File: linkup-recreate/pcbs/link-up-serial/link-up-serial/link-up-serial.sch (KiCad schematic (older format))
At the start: 6 parts

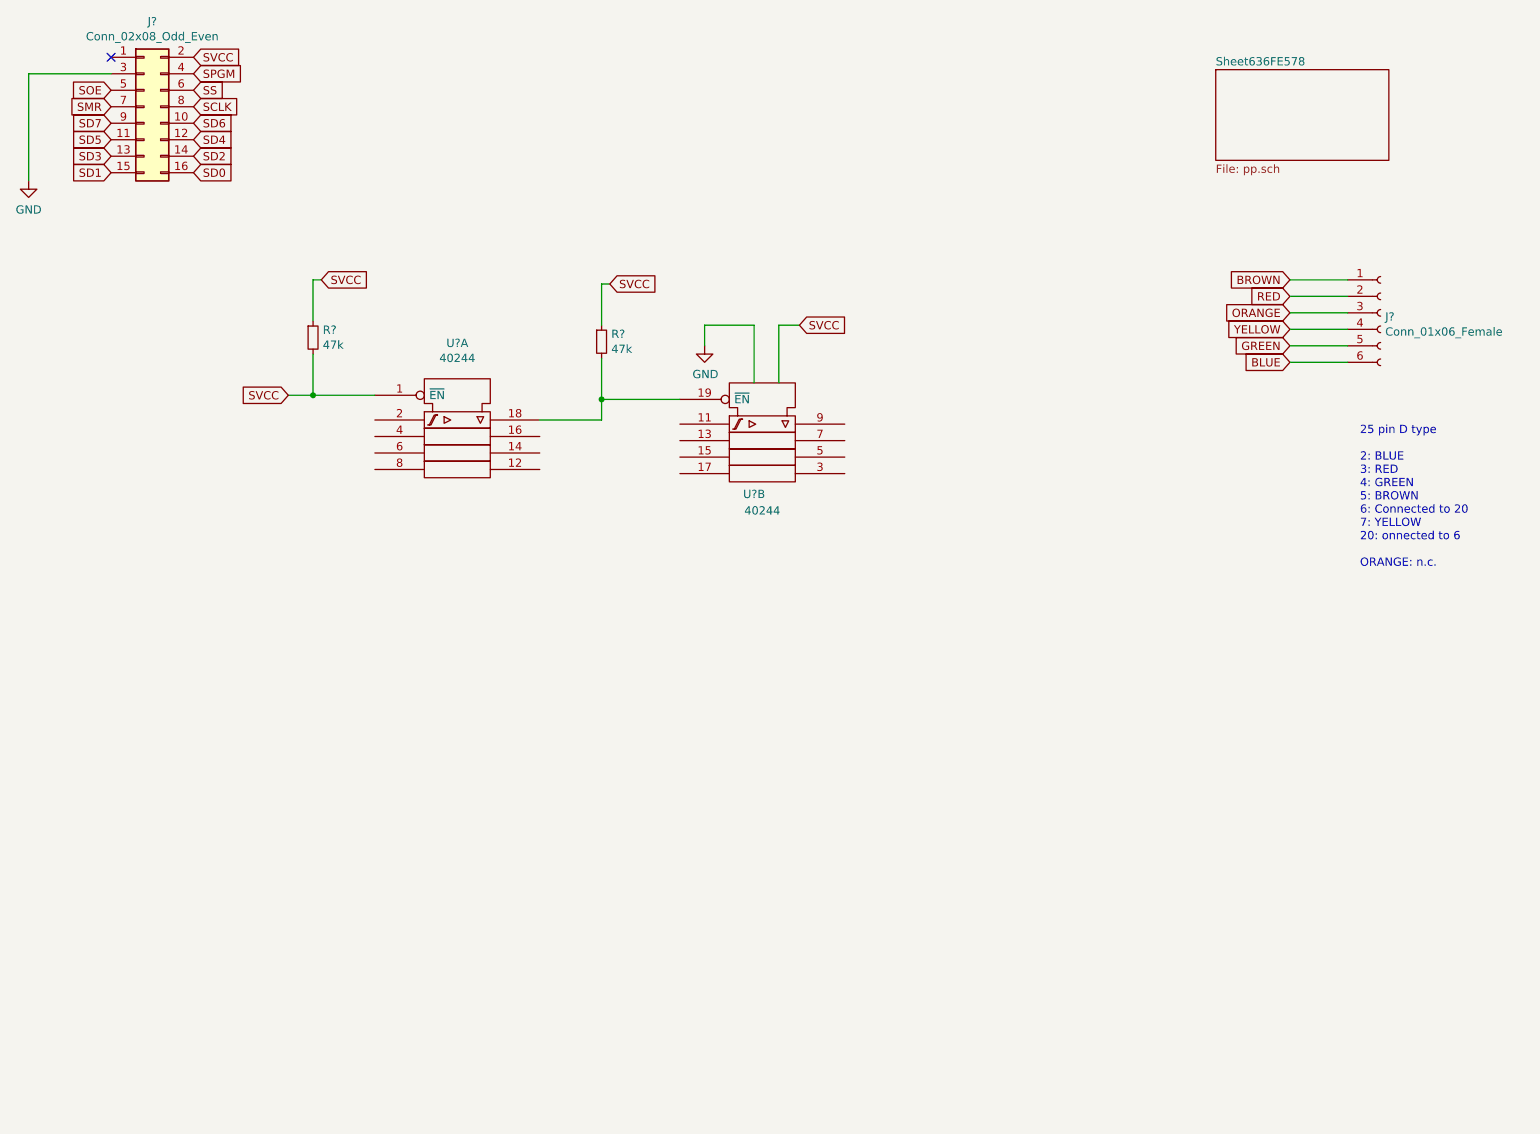
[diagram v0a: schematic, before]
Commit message: Updates
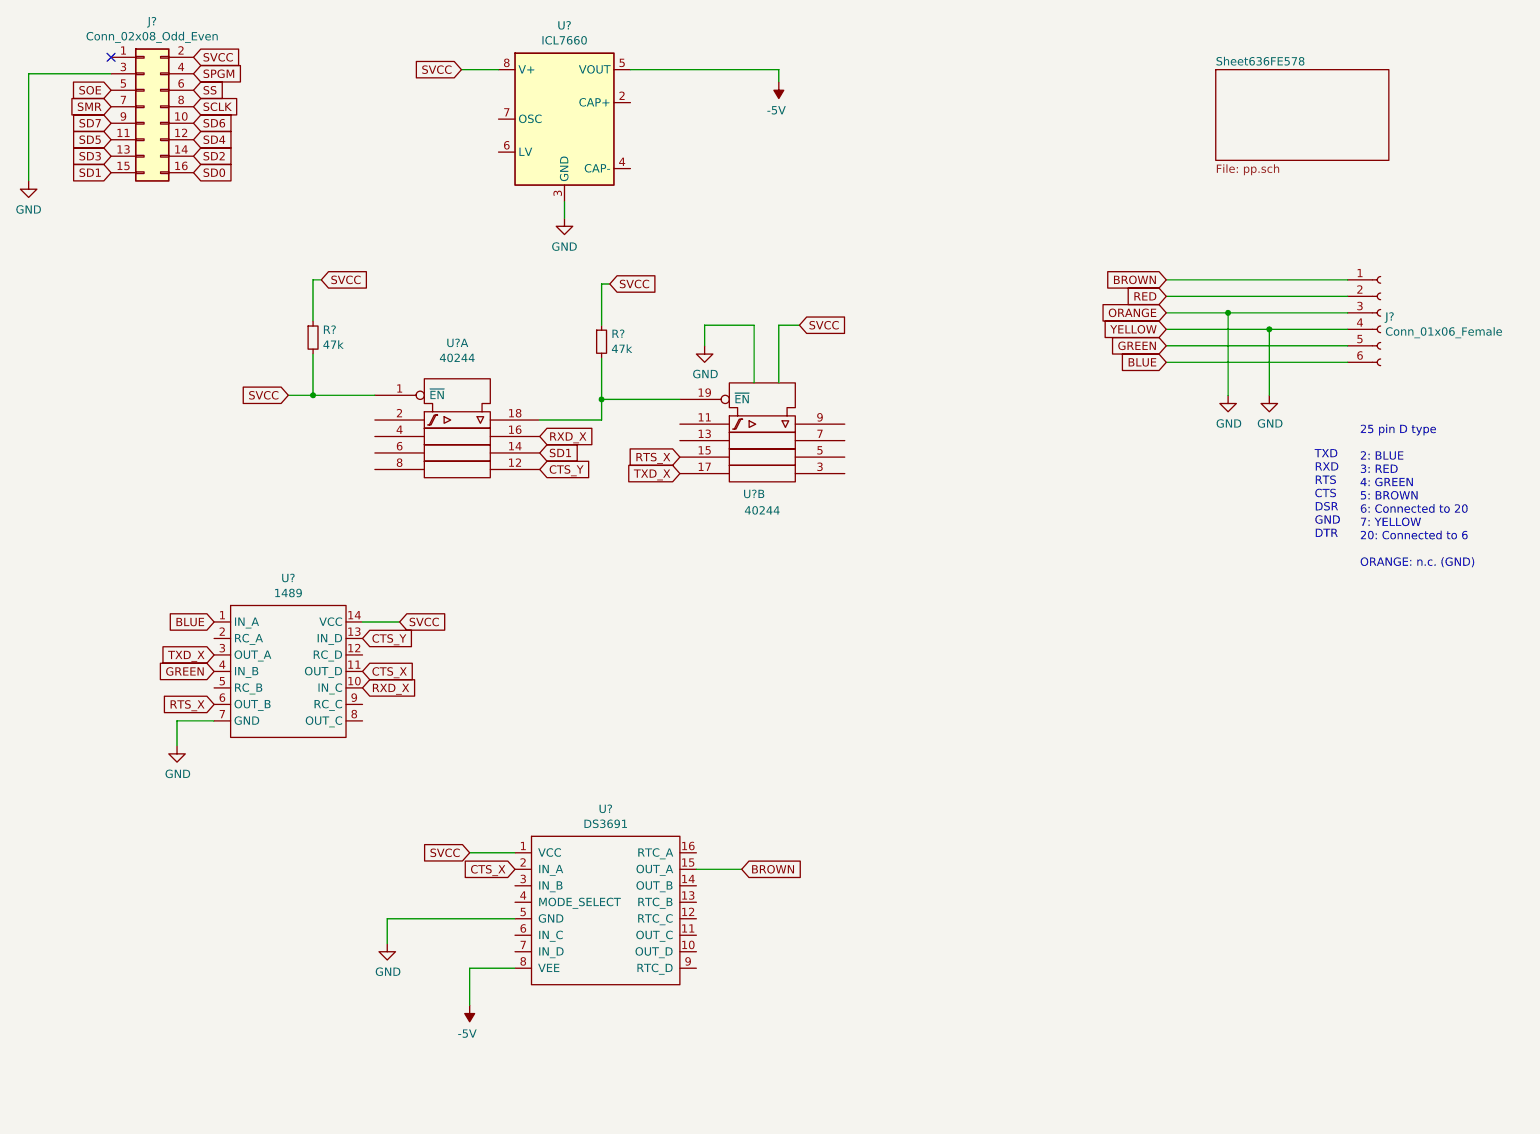
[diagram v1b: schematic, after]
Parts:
- added U?: 1489, symbol ajm:1489
- added U?: DS3691, symbol ajm:DS3691
- added U?: ICL7660, symbol Regulator_SwitchedCapacitor:ICL7660
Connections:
- net ORANGE is gone; now on net GND: J?.3 (Pin_3)
- net YELLOW is gone; now on net GND: J?.4 (Pin_4)
- net BLUE: now also U?.1 (IN_A)
- net BROWN: now also U?.15 (OUT_A)
- net GND: now also U?.3 (GND), U?.5 (GND), U?.7 (GND)
- net GREEN: now also U?.4 (IN_B)
- net SD1: now also U?.14
- net Vdd: now also U?.1 (VCC), U?.14 (VCC), U?.8 (V+)
- net CTS_Y: now reaches U?.12
- net CTS_Y: now also U?.13 (IN_D)
- net RXD_X: now reaches U?.16
- net RXD_X: now also U?.10 (IN_C)
- net RTS_X: now reaches U?.15
- net RTS_X: now also U?.6 (OUT_B)
- net TXD_X: now reaches U?.17
- net TXD_X: now also U?.3 (OUT_A)
- new net -5V: U?.5 (VOUT), U?.8 (VEE)
- new net CTS_X: U?.11 (OUT_D), U?.2 (IN_A)
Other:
- note added: "25 pin D type\n\n2: BLUE\n3: RED\n4: GREEN\n5: BROWN\n6: Connected to 20\n7: YELLOW\n20: Connected to 6\n\nORANGE: n.c. (GND)\n"
- note added: "TXD\nRXD\nRTS\nCTS\nDSR\nGND\nDTR"
- note removed: "25 pin D type\n\n2: BLUE\n3: RED\n4: GREEN\n5: BROWN\n6: Connected to 20\n7: YELLOW\n20: onnected to 6\n\nORANGE: n.c.\n"
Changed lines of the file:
@@
 Wire Wire Line
 	2700 2425 2750 2425
-Text GLabel 8625 2425 0    50   Input ~ 0
+Text GLabel 7875 2425 0    50   Input ~ 0
 BROWN
-Text GLabel 8625 2525 0    50   Input ~ 0
+Text GLabel 7875 2525 0    50   Input ~ 0
 RED
-Text GLabel 8625 2625 0    50   Input ~ 0
+Text GLabel 7875 2625 0    50   Input ~ 0
 ORANGE
-Text GLabel 8625 2725 0    50   Input ~ 0
+Text GLabel 7875 2725 0    50   Input ~ 0
 YELLOW
-Text GLabel 8625 2825 0    50   Input ~ 0
+Text GLabel 7875 2825 0    50   Input ~ 0
 GREEN
-Text GLabel 8625 2925 0    50   Input ~ 0
+Text GLabel 7875 2925 0    50   Input ~ 0
 BLUE
 $Comp
@@
 $EndComp
 Wire Wire Line
-	8975 2425 8625 2425
-Wire Wire Line
-	8625 2525 8975 2525
-Wire Wire Line
-	8975 2625 8625 2625
-Wire Wire Line
-	8625 2725 8975 2725
-Wire Wire Line
-	8625 2825 8975 2825
-Wire Wire Line
-	8625 2925 8975 2925
+	8975 2425 7875 2425
+Wire Wire Line
+	7875 2525 8975 2525
+Wire Wire Line
+	8975 2625 8250 2625
+Wire Wire Line
+	7875 2725 8500 2725
+Wire Wire Line
+	7875 2825 8975 2825
+Wire Wire Line
+	7875 2925 8975 2925
 Text Notes 9050 4175 0    50   ~ 0
-25 pin D type\n\n2: BLUE\n3: RED\n4: GREEN\n5: BROWN\n6: Connected to 20\n7: YELLOW\n20: onnected to 6\n\nORANGE: n.c.\n
+25 pin D type\n\n2: BLUE\n3: RED\n4: GREEN\n5: BROWN\n6: Connected to 20\n7: YELLOW\n20: Connected to 6\n\nORANGE: n.c. (GND)\n
 Wire Wire Line
 	4075 3275 4450 3275
@@
 	4925 3150 4450 3150
 Connection ~ 4450 3150
+$Comp
+L ajm:1489 U?
+U 1 1 6371CD69
+P 2050 4400
+F 0 "U?" H 2550 4565 50  0000 C CNN
+F 1 "1489" H 2550 4474 50  0000 C CNN
+F 2 "" H 2050 4400 50  0001 C CNN
+F 3 "" H 2050 4400 50  0001 C CNN
+	1    2050 4400
+	1    0    0    -1
+$EndComp
+$Comp
+L ajm:DS3691 U?
+U 1 1 6371DF57
+P 4025 5800
+F 0 "U?" H 4475 5965 50  0000 C CNN
+F 1 "DS3691" H 4475 5874 50  0000 C CNN
+F 2 "" H 4025 5800 50  0001 C CNN
+F 3 "" H 4025 5800 50  0001 C CNN
+	1    4025 5800
+	1    0    0    -1
+$EndComp
+$Comp
+L Regulator_SwitchedCapacitor:ICL7660 U?
+U 1 1 6371F6A3
+P 4225 1450
+F 0 "U?" H 4225 2017 50  0000 C CNN
+F 1 "ICL7660" H 4225 1926 50  0000 C CNN
+F 2 "" H 4325 1350 50  0001 C CNN
+F 3 "http://datasheets.maximintegrated.com/en/ds/ICL7660-MAX1044.pdf" H 4325 1350 50  0001 C CNN
+	1    4225 1450
+	1    0    0    -1
+$EndComp
+Text GLabel 3600 1150 0    50   Input ~ 0
+SVCC
+Wire Wire Line
+	3600 1150 3825 1150
+$Comp
+L power:GND #PWR?
+U 1 1 63721337
+P 4225 2050
+AR Path="/6104FF77/63721337" Ref="#PWR?"  Part="1"
+AR Path="/63721337" Ref="#PWR?"  Part="1"
+AR Path="/636FE579/63721337" Ref="#PWR?"  Part="1"
+F 0 "#PWR?" H 4225 1800 50  0001 C CNN
+F 1 "GND" H 4225 1875 50  0000 C CNN
+F 2 "" H 4225 2050 50  0001 C CNN
+F 3 "" H 4225 2050 50  0001 C CNN
+	1    4225 2050
+	1    0    0    -1
+$EndComp
+Wire Wire Line
+	4225 2050 4225 1950
+$Comp
+L power:-5V #PWR?
+U 1 1 63721F90
+P 5525 1225
+F 0 "#PWR?" H 5525 1325 50  0001 C CNN
+F 1 "-5V" H 5540 1398 50  0000 C CNN
+F 2 "" H 5525 1225 50  0001 C CNN
+F 3 "" H 5525 1225 50  0001 C CNN
+	1    5525 1225
+	-1   0    0    1
+$EndComp
+$Comp
+L power:-5V #PWR?
+U 1 1 63722CFC
+P 3650 6825
+F 0 "#PWR?" H 3650 6925 50  0001 C CNN
+F 1 "-5V" H 3665 6998 50  0000 C CNN
+F 2 "" H 3650 6825 50  0001 C CNN
+F 3 "" H 3650 6825 50  0001 C CNN
+	1    3650 6825
+	-1   0    0    1
+$EndComp
+Wire Wire Line
+	3925 6600 3650 6600
+Wire Wire Line
+	3650 6600 3650 6825
+Wire Wire Line
+	5525 1150 5525 1225
+Wire Wire Line
+	4625 1150 5525 1150
+Wire Wire Line
+	3925 5900 3650 5900
+$Comp
+L power:GND #PWR?
+U 1 1 63725A73
+P 3150 6450
+F 0 "#PWR?" H 3150 6200 50  0001 C CNN
+F 1 "GND" H 3155 6277 50  0000 C CNN
+F 2 "" H 3150 6450 50  0001 C CNN
+F 3 "" H 3150 6450 50  0001 C CNN
+	1    3150 6450
+	1    0    0    -1
+$EndComp
+Wire Wire Line
+	3925 6300 3150 6300
+Wire Wire Line
+	3150 6300 3150 6450
+Text GLabel 5300 6000 2    50   Input ~ 0
+BROWN
+Wire Wire Line
+	5300 6000 5025 6000
+Text GLabel 4925 3600 0    50   Input ~ 0
+TXD_X
+Text GLabel 2100 4700 0    50   Input ~ 0
+TXD_X
+$Comp
+L power:GND #PWR?
+U 1 1 63727763
+P 1875 5250
+F 0 "#PWR?" H 1875 5000 50  0001 C CNN
+F 1 "GND" H 1880 5077 50  0000 C CNN
+F 2 "" H 1875 5250 50  0001 C CNN
+F 3 "" H 1875 5250 50  0001 C CNN
+	1    1875 5250
+	1    0    0    -1
+$EndComp
+Wire Wire Line
+	2100 5100 1875 5100
+Wire Wire Line
+	1875 5100 1875 5250
+Text GLabel 3650 5900 0    50   Input ~ 0
+SVCC
+Text GLabel 3225 4500 2    50   Input ~ 0
+SVCC
+Wire Wire Line
+	3000 4500 3225 4500
+Text GLabel 2100 4500 0    50   Input ~ 0
+BLUE
+Text Notes 8775 4000 0    50   ~ 0
+TXD\nRXD\nRTS\nCTS\nDSR\nGND\nDTR
+$Comp
+L power:GND #PWR?
+U 1 1 6372AA19
+P 8250 3125
+F 0 "#PWR?" H 8250 2875 50  0001 C CNN
+F 1 "GND" H 8255 2952 50  0000 C CNN
+F 2 "" H 8250 3125 50  0001 C CNN
+F 3 "" H 8250 3125 50  0001 C CNN
+	1    8250 3125
+	1    0    0    -1
+$EndComp
+Wire Wire Line
+	8250 3125 8250 2625
+Connection ~ 8250 2625
+Wire Wire Line
+	8250 2625 7875 2625
+$Comp
+L power:GND #PWR?
+U 1 1 6372B87A
+P 8500 3125
+F 0 "#PWR?" H 8500 2875 50  0001 C CNN
+F 1 "GND" H 8505 2952 50  0000 C CNN
+F 2 "" H 8500 3125 50  0001 C CNN
+F 3 "" H 8500 3125 50  0001 C CNN
+	1    8500 3125
+	1    0    0    -1
+$EndComp
+Wire Wire Line
+	8500 3125 8500 2725
+Connection ~ 8500 2725
+Wire Wire Line
+	8500 2725 8975 2725
+Text GLabel 4075 3375 2    50   Input ~ 0
+RXD_X
+Text GLabel 3000 4900 2    50   Input ~ 0
+RXD_X
+Text GLabel 2100 4800 0    50   Input ~ 0
+GREEN
+Text GLabel 2100 5000 0    50   Input ~ 0
+RTS_X
+Text GLabel 4925 3500 0    50   Input ~ 0
+RTS_X
+Text GLabel 4075 3475 2    50   Input ~ 0
+SD1
+Text GLabel 4075 3575 2    50   Input ~ 0
+CTS_Y
+Text GLabel 3000 4800 2    50   Input ~ 0
+CTS_X
+Text GLabel 3925 6000 0    50   Input ~ 0
+CTS_X
+Text GLabel 3000 4600 2    50   Input ~ 0
+CTS_Y
 $EndSCHEMATC

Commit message: Updates
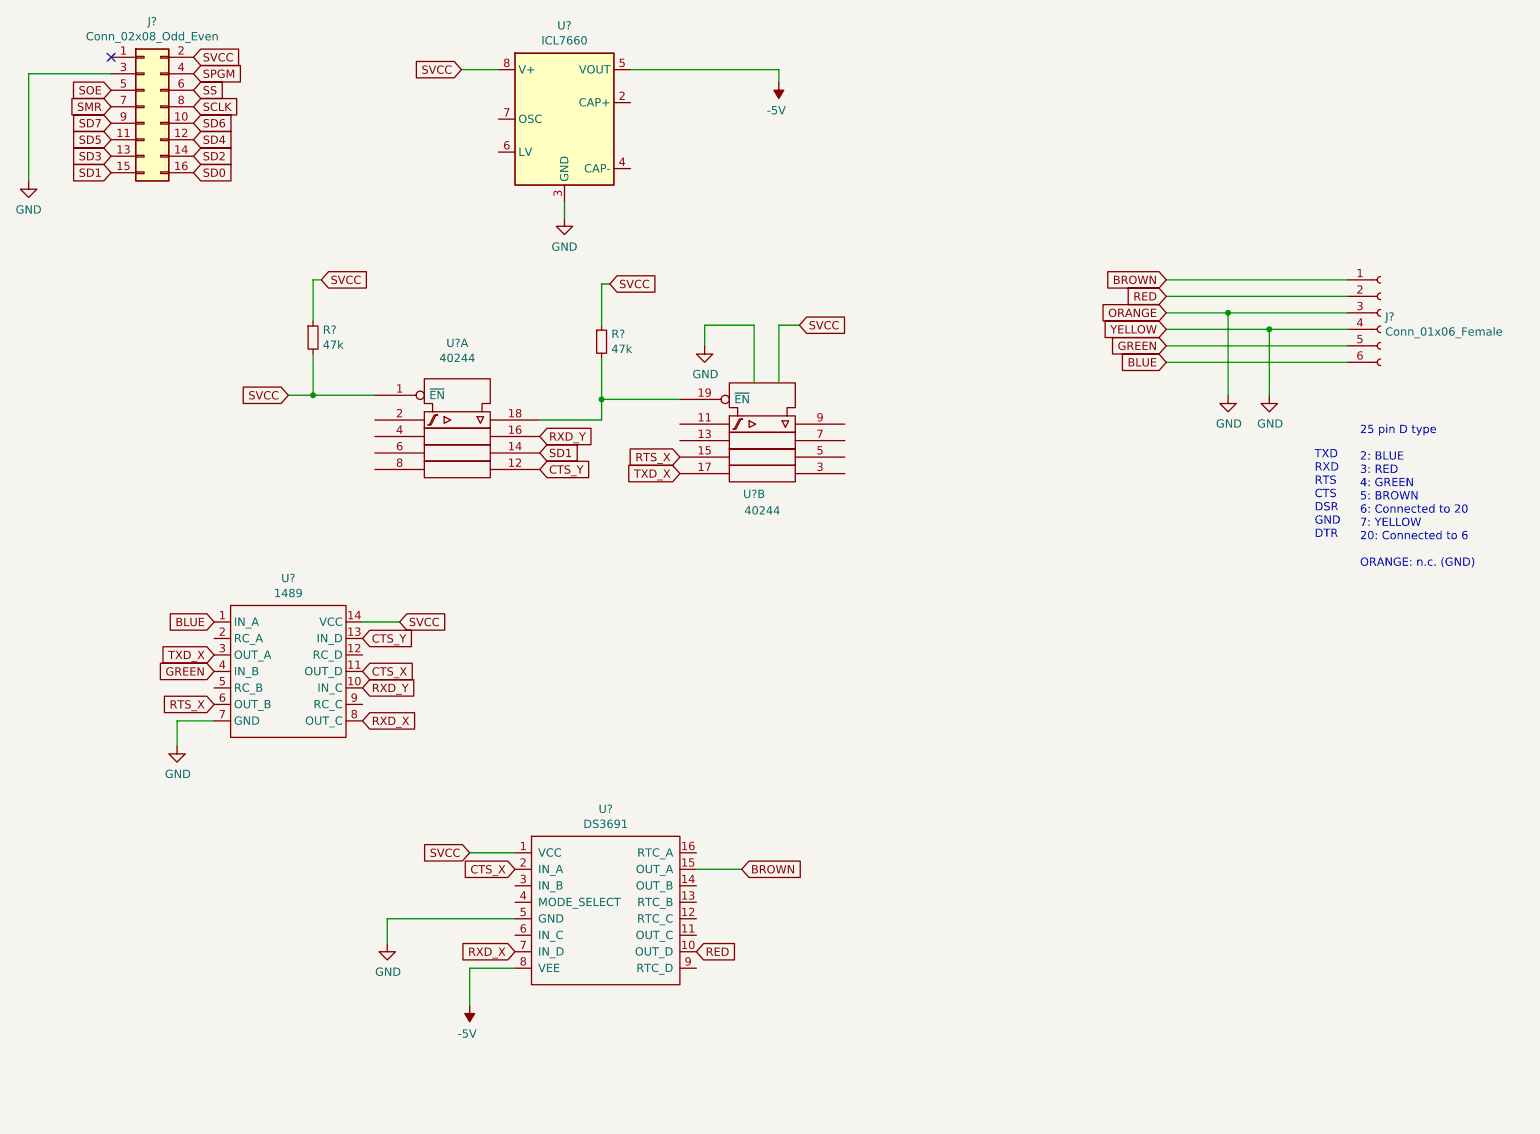
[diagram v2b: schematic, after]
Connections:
- net RED: now also U?.10 (OUT_D)
- net RXD_X: now also U?.7 (IN_D), U?.8 (OUT_C); no longer U?.10 (IN_C), U?.16
- new net RXD_Y: U?.10 (IN_C), U?.16
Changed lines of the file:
@@
 $Descr A4 11693 8268
 encoding utf-8
-Sheet 1 2
+Sheet 1 1
 Title ""
 Date ""
@@
 Comment4 ""
 $EndDescr
-$Sheet
-S 8175 1150 1050 550
-U 636FE579
-F0 "Sheet636FE578" 50
-F1 "pp.sch" 50
-$EndSheet
 Text GLabel 1475 1775 0    50   Input ~ 0
 SD1
@@
 	8500 2725 8975 2725
 Text GLabel 4075 3375 2    50   Input ~ 0
-RXD_X
+RXD_Y
 Text GLabel 3000 4900 2    50   Input ~ 0
-RXD_X
+RXD_Y
 Text GLabel 2100 4800 0    50   Input ~ 0
 GREEN
@@
 Text GLabel 3000 4600 2    50   Input ~ 0
 CTS_Y
+Text GLabel 3000 5100 2    50   Input ~ 0
+RXD_X
+Text GLabel 3925 6500 0    50   Input ~ 0
+RXD_X
+Text GLabel 5025 6500 2    50   Input ~ 0
+RED
 $EndSCHEMATC

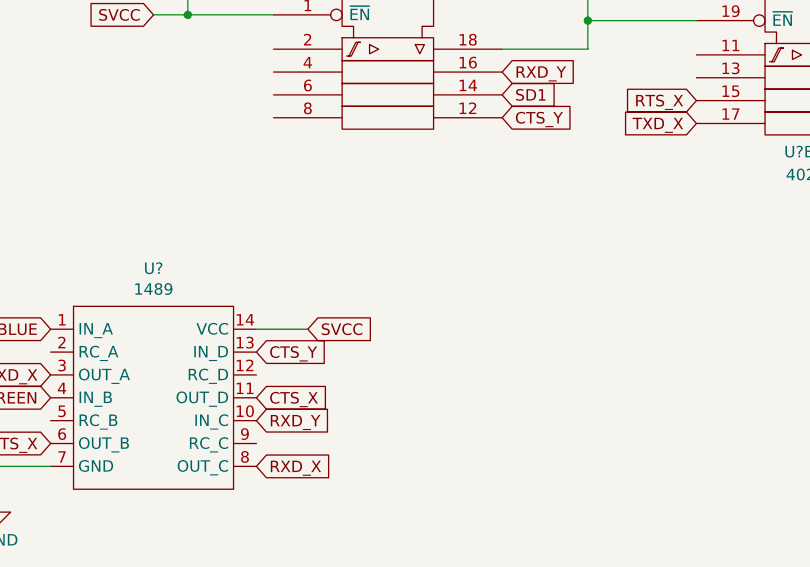
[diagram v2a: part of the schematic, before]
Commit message: Updates
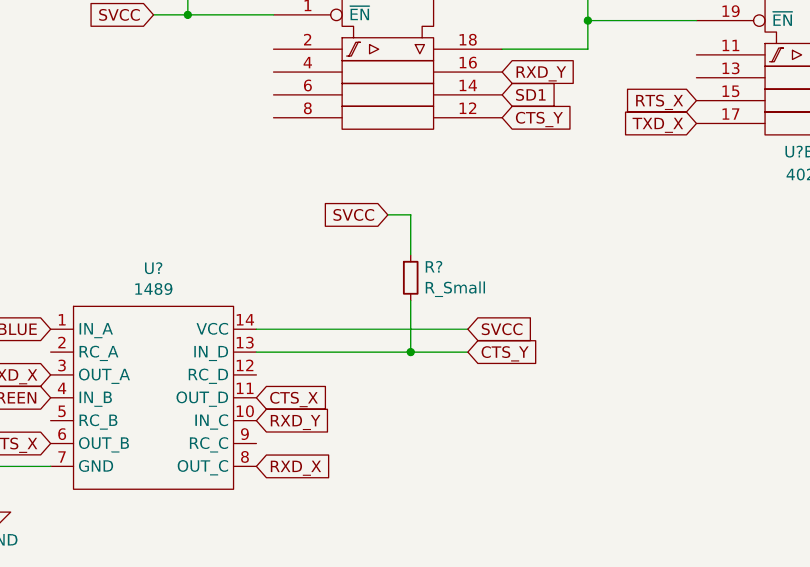
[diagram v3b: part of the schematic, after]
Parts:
- added R?: R_Small, symbol Device:R_Small
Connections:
- net CTS_Y: now also R?.2
- net Vdd: now also R?.1
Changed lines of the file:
@@
 Text GLabel 3650 5900 0    50   Input ~ 0
 SVCC
-Text GLabel 3225 4500 2    50   Input ~ 0
+Text GLabel 3925 4500 2    50   Input ~ 0
 SVCC
-Wire Wire Line
-	3000 4500 3225 4500
 Text GLabel 2100 4500 0    50   Input ~ 0
 BLUE
@@
 Text GLabel 3925 6000 0    50   Input ~ 0
 CTS_X
-Text GLabel 3000 4600 2    50   Input ~ 0
+Text GLabel 3925 4600 2    50   Input ~ 0
 CTS_Y
 Text GLabel 3000 5100 2    50   Input ~ 0
@@
 Text GLabel 5025 6500 2    50   Input ~ 0
 RED
+Wire Wire Line
+	3000 4600 3675 4600
+Wire Wire Line
+	3000 4500 3925 4500
+$Comp
+L Device:R_Small R?
+U 1 1 637324DD
+P 3675 4275
+F 0 "R?" H 3734 4321 50  0000 L CNN
+F 1 "R_Small" H 3734 4230 50  0000 L CNN
+F 2 "" H 3675 4275 50  0001 C CNN
+F 3 "~" H 3675 4275 50  0001 C CNN
+	1    3675 4275
+	1    0    0    -1
+$EndComp
+Text GLabel 3575 4000 0    50   Input ~ 0
+SVCC
+Wire Wire Line
+	3575 4000 3675 4000
+Wire Wire Line
+	3675 4000 3675 4175
+Wire Wire Line
+	3675 4375 3675 4600
+Connection ~ 3675 4600
+Wire Wire Line
+	3675 4600 3925 4600
 $EndSCHEMATC
